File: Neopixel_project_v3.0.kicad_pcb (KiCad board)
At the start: 2 copper layers, 50 x 50 mm, 64 parts, among them J1 Conn_01x03_Pin, J3 Screw_Terminal_01x02, Q1 MMBT3904, Q2 MMBT3904, Q3 MMBT3904, Q4 MMBT3904, Q5 DO3407B, Q6 DO3407B, Q7 DO3407B, Q8 DO3407B, SW1 TS-1088-AR02016, SW2 TS-1088-AR02016, U1 ESP8685H4, U2 AL8843, U3 TD1469, U4 USBLC6-4SC6, Y1 Crystal_GND24

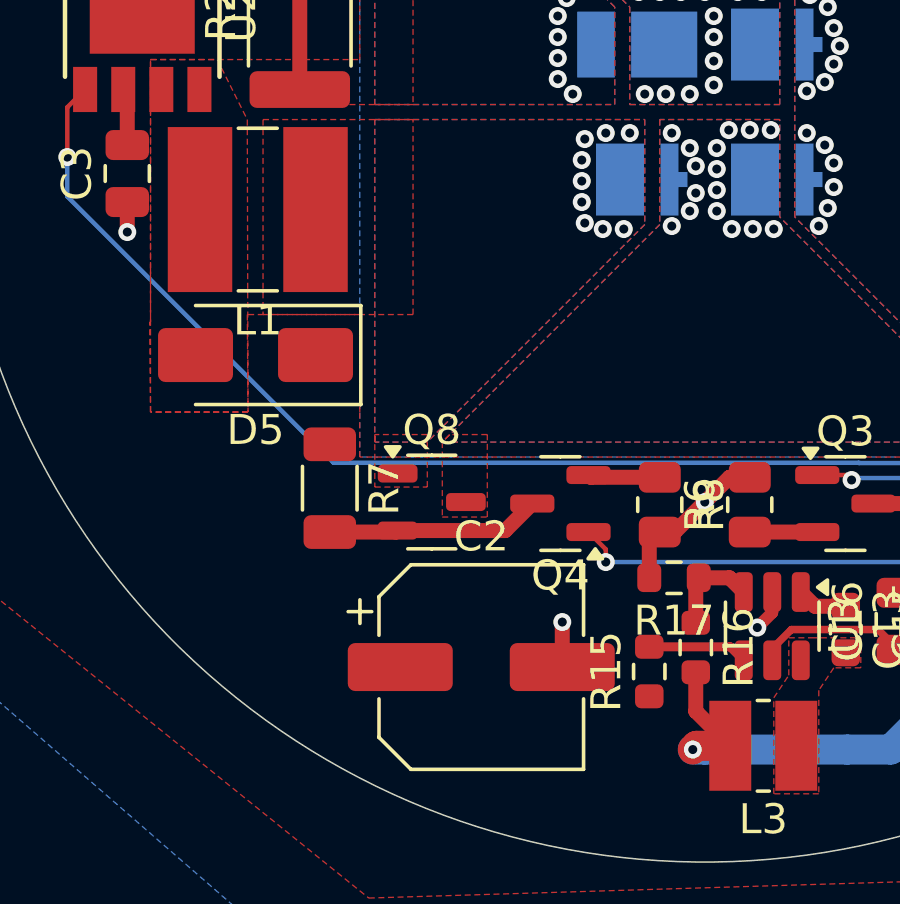
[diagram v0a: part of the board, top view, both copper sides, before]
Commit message: added bom.csv and buch of other changes
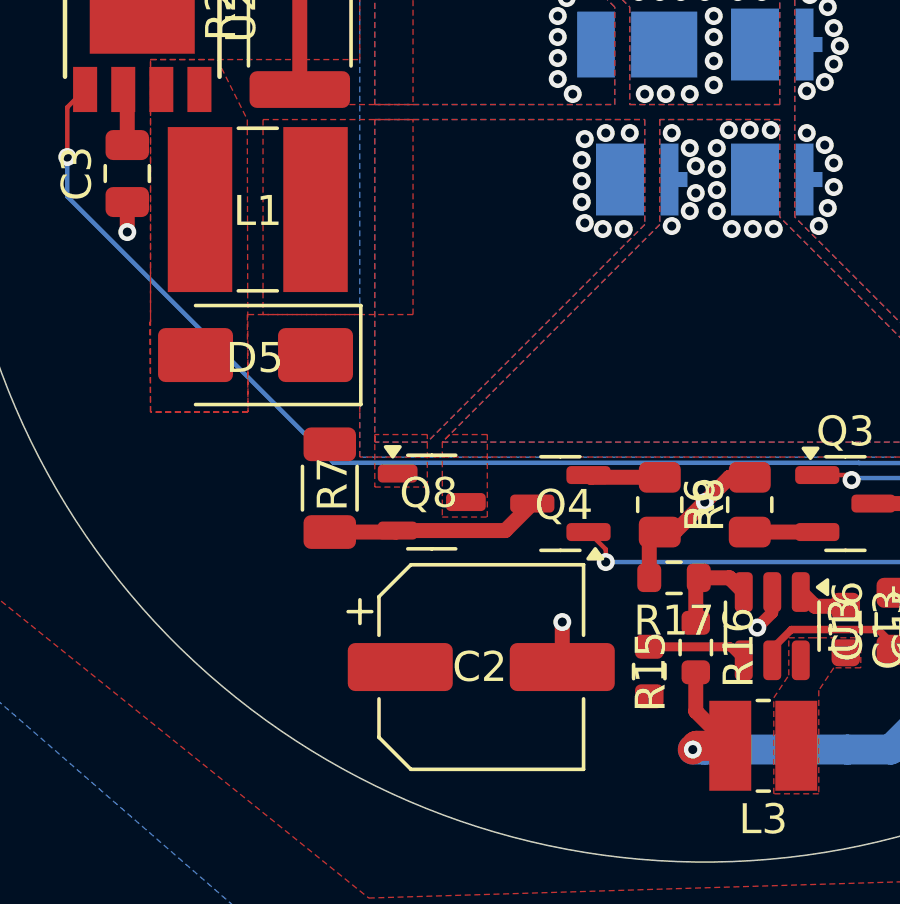
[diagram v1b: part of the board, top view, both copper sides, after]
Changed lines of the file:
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@@
 		(tags "SOT TO_SOT_SMD")
 		(property "Reference" "Q4"
-			(at 0 -2.4 180)
+			(at -0.1125 -0.05 180)
 			(layer "F.SilkS")
 			(effects
@@
 		(tags "SOT TO_SOT_SMD")
 		(property "Reference" "Q8"
-			(at 0 -2.4 0)
+			(at -0.1 -0.3 0)
 			(layer "F.SilkS")
 			(effects
@@
 		(tags "Diode SMA (DO-214AC)")
 		(property "Reference" "D5"
-			(at 0 -2.5 180)
+			(at 0.025 -0.1 180)
 			(layer "F.SilkS")
 			(effects
@@
 		(tags "resistor")
 		(property "Reference" "R7"
-			(at 0 -1.82 90)
+			(at -0.1375 -0.1 90)
 			(layer "F.SilkS")
 			(effects
@@
 		(tags "resistor")
 		(property "Reference" "R15"
-			(at 0 -1.43 270)
+			(at 0 0.05 270)
 			(layer "F.SilkS")
 			(effects
@@
 		(tags "smd inductor dlg-0504")
 		(property "Reference" "L1"
-			(at 0 -3.7 180)
+			(at 0 -0.05 180)
 			(layer "F.SilkS")
 			(effects
@@
 		(tags "capacitor electrolytic")
 		(property "Reference" "C2"
-			(at 0 -4.35 360)
+			(at -0.05 0 360)
 			(layer "F.SilkS")
 			(effects
@@
 		(layer "User.1")
 	)
-	(gr_circle
-		(center 201 141)
-		(end 228.5 141)
-		(stroke
-			(width 0.1)
-			(type default)
-		)
-		(fill none)
-		(layer "User.2")
-	)
 	(dimension
